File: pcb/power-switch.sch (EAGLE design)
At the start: 22 parts, among them CON1 KF301-3P, CON2 KF301-3P, K1 SMIH-12VDC-S-L-C, K2 SMIH-12VDC-S-L-C, U1 MCP1631X, U6 EFM32PG1B200_Q32, U7 RFM69HW

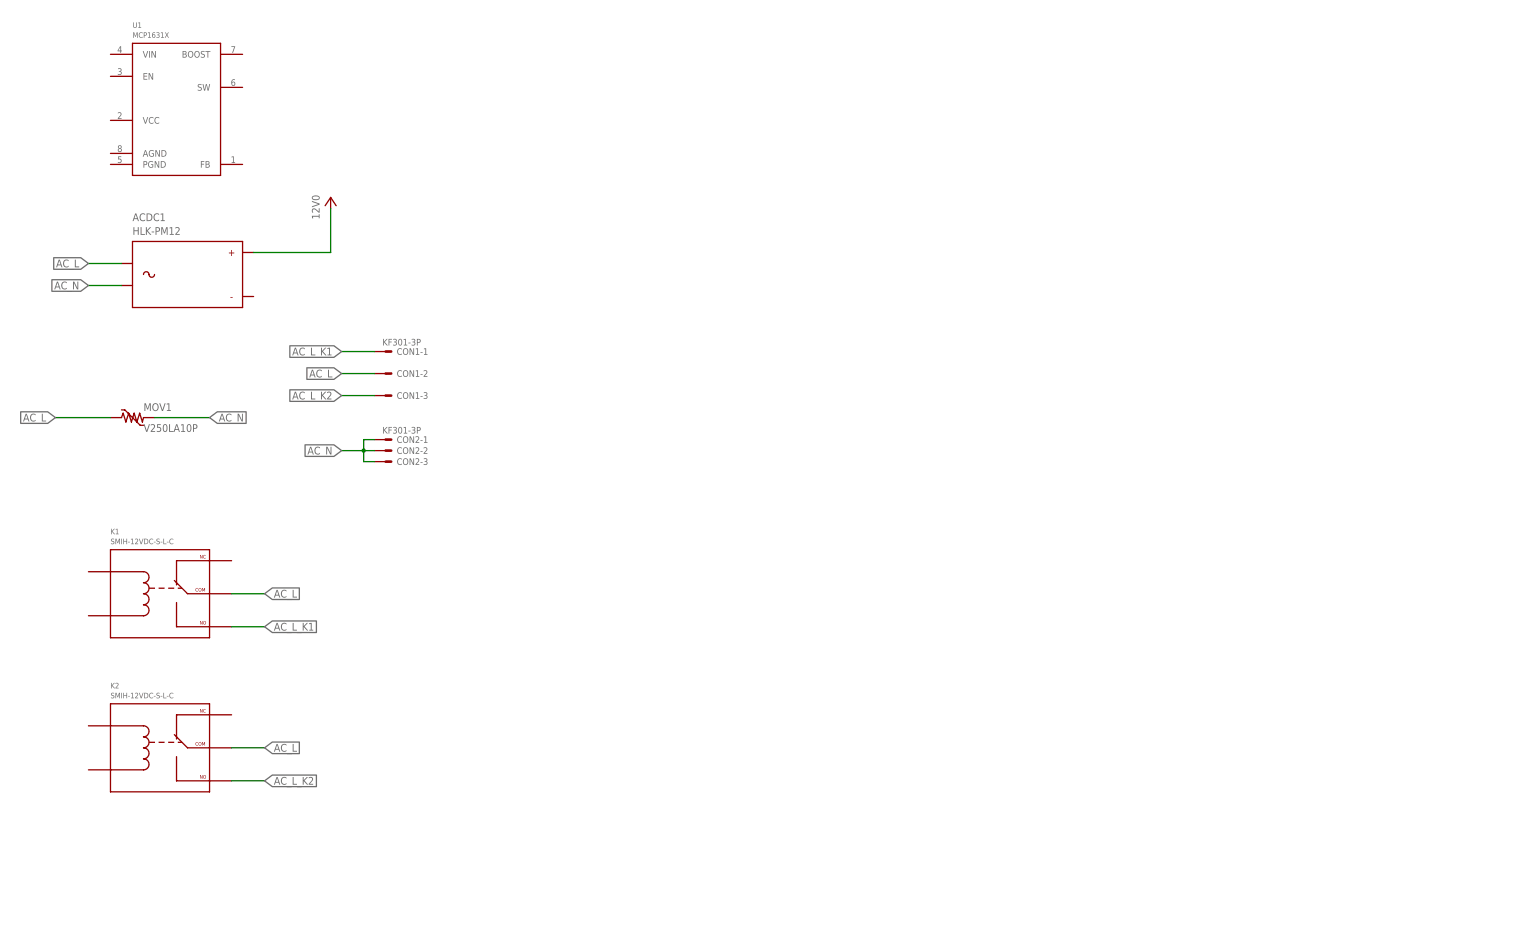
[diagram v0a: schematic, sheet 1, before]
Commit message: PCB Work
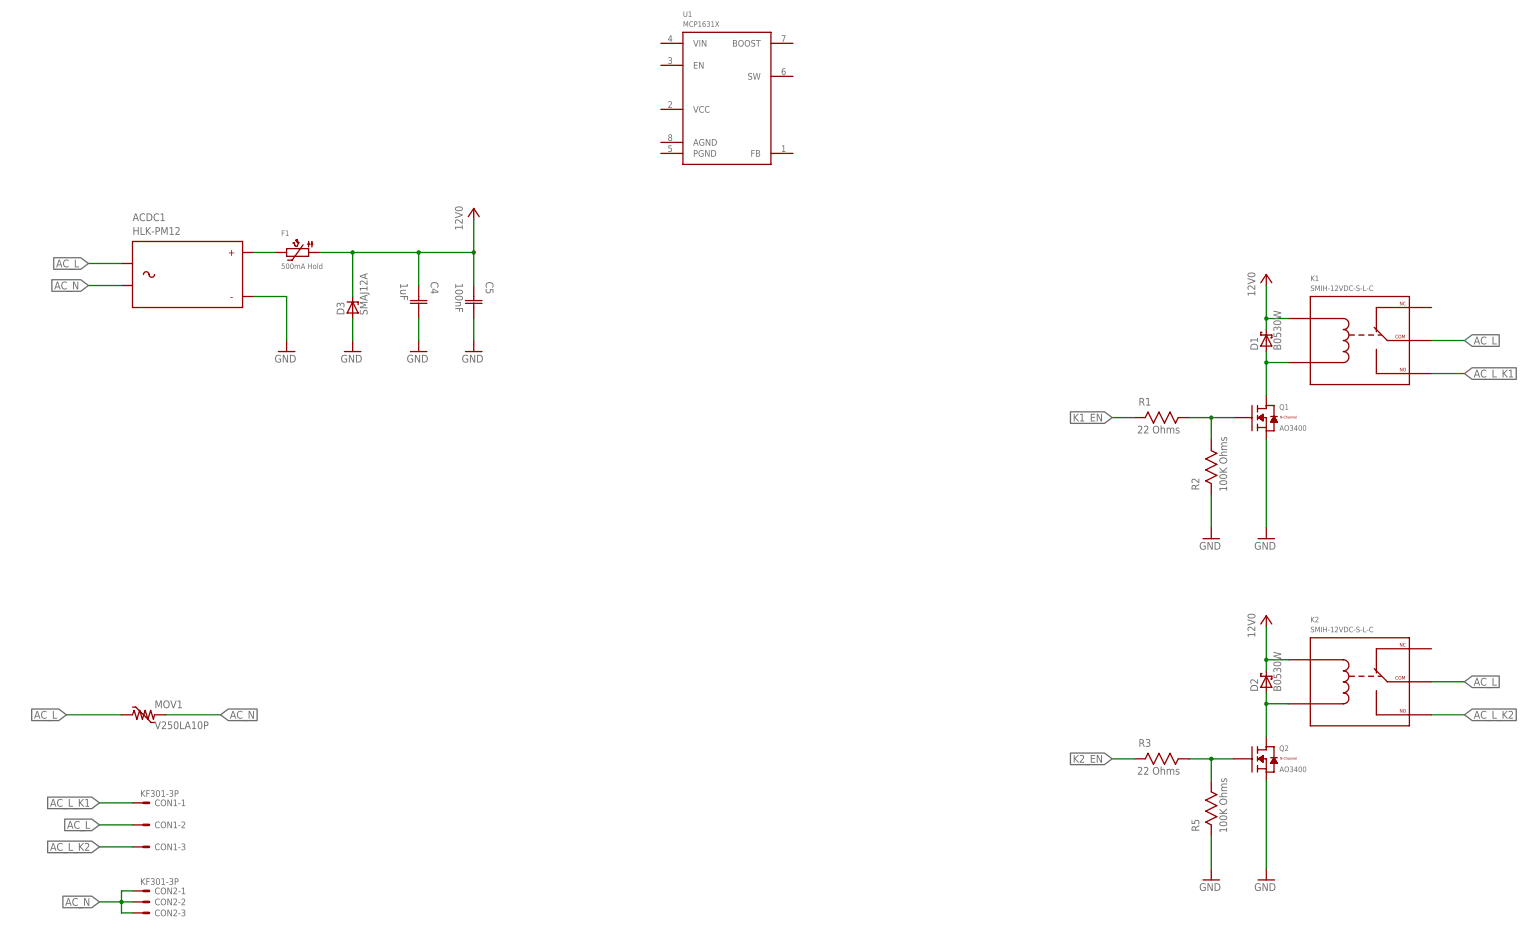
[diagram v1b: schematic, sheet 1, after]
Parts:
- added C4: 1uF, Capacitor:CAPACITOR-1206
- added C5: 100nF, Capacitor:CAPACITOR-0603
- added D1, D2: B0530W, Generic Diode:B0530W
- added D3: SMAJ12A, TVS:SMAJ12A
- added F1: 500mA Hold, PTC Fuses:PTC1812
- added Q1, Q2: AO3400, Alpha Omega:AO3400
- added R1, R3: 22 Ohms, Resistor:RESISTOR-0603
- added R2, R5: 100K Ohms, Resistor:RESISTOR-0603
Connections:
- new net K1_EN: R1.2
- new net K2_EN: R3.2
- new net N$2: Q1.G, R1.1, R2.1
- new net N$3: D1.A, K1.COIL2, Q1.D
- new net N$4: Q2.G, R3.1, R5.1
- new net N$5: D2.A, K2.COIL2, Q2.D
- new net N$7: ACDC1.+VO, F1.2
- net 12V0: now also C4.C1, C5.C1, D1.C, D2.C, D3.C, F1.1, K1.COIL1, K2.COIL1; no longer ACDC1.+VO
- net GND: now also ACDC1.-VO, C4.C2, C5.C2, D3.A, Q1.S, Q2.S, R2.2, R5.2
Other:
- moved on the sheet: CON1-1, CON1-2, CON1-3, CON2-1, CON2-2, CON2-3, K1, K2, MOV1, U1
